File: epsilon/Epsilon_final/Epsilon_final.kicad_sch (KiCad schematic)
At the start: 16 parts, among them J3 Conn_01x02_Pin, J4 Conn_01x02_Pin, Q5 AO3401A, U12 ADA4940-1ARZ-R7, U8 DS28E07P+T

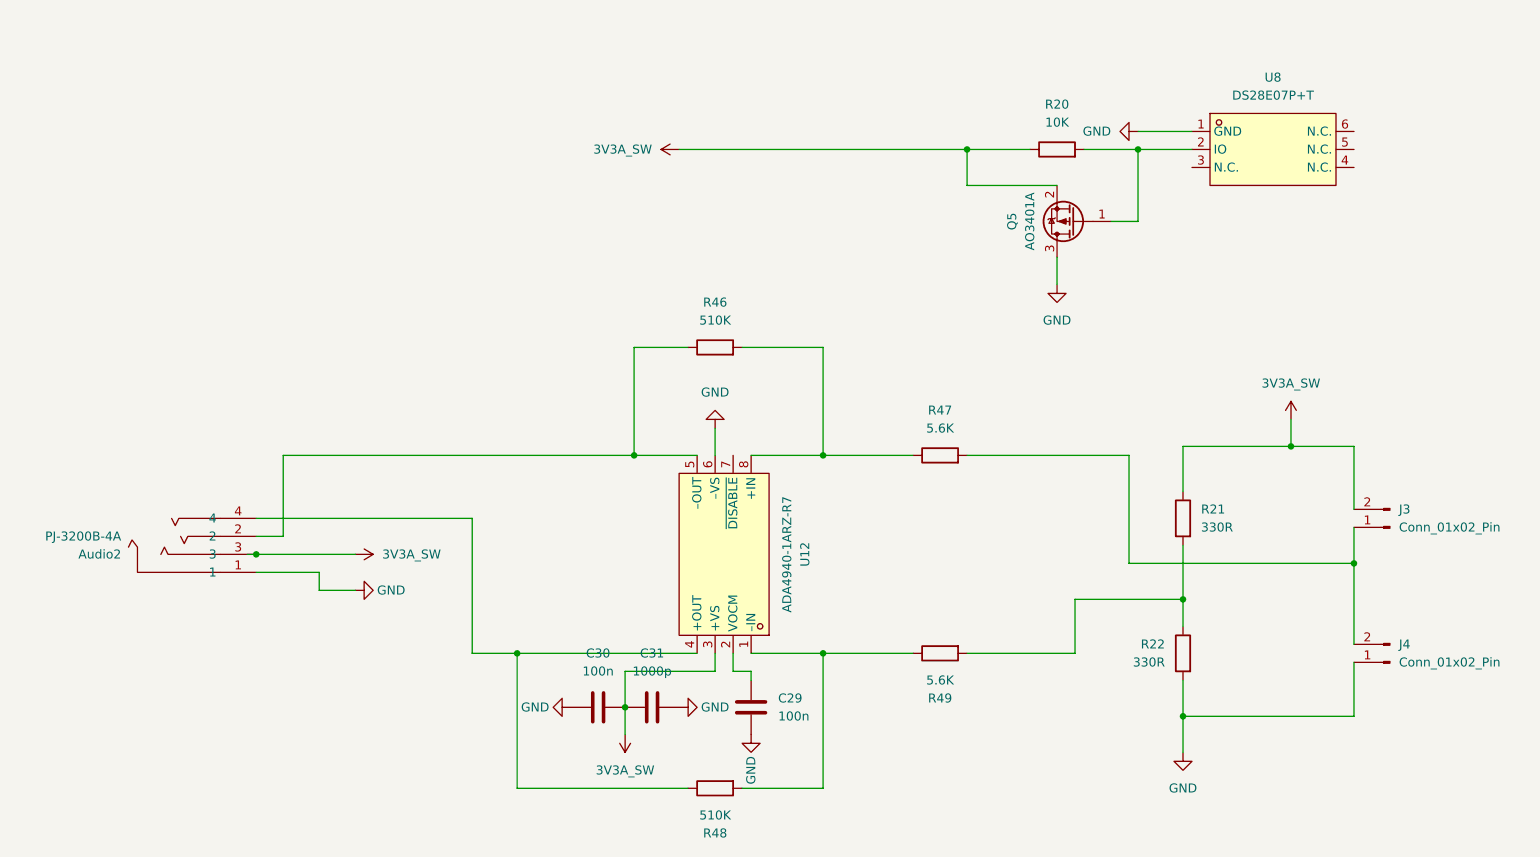
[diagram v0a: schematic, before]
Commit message: Yolo2
new Ozys
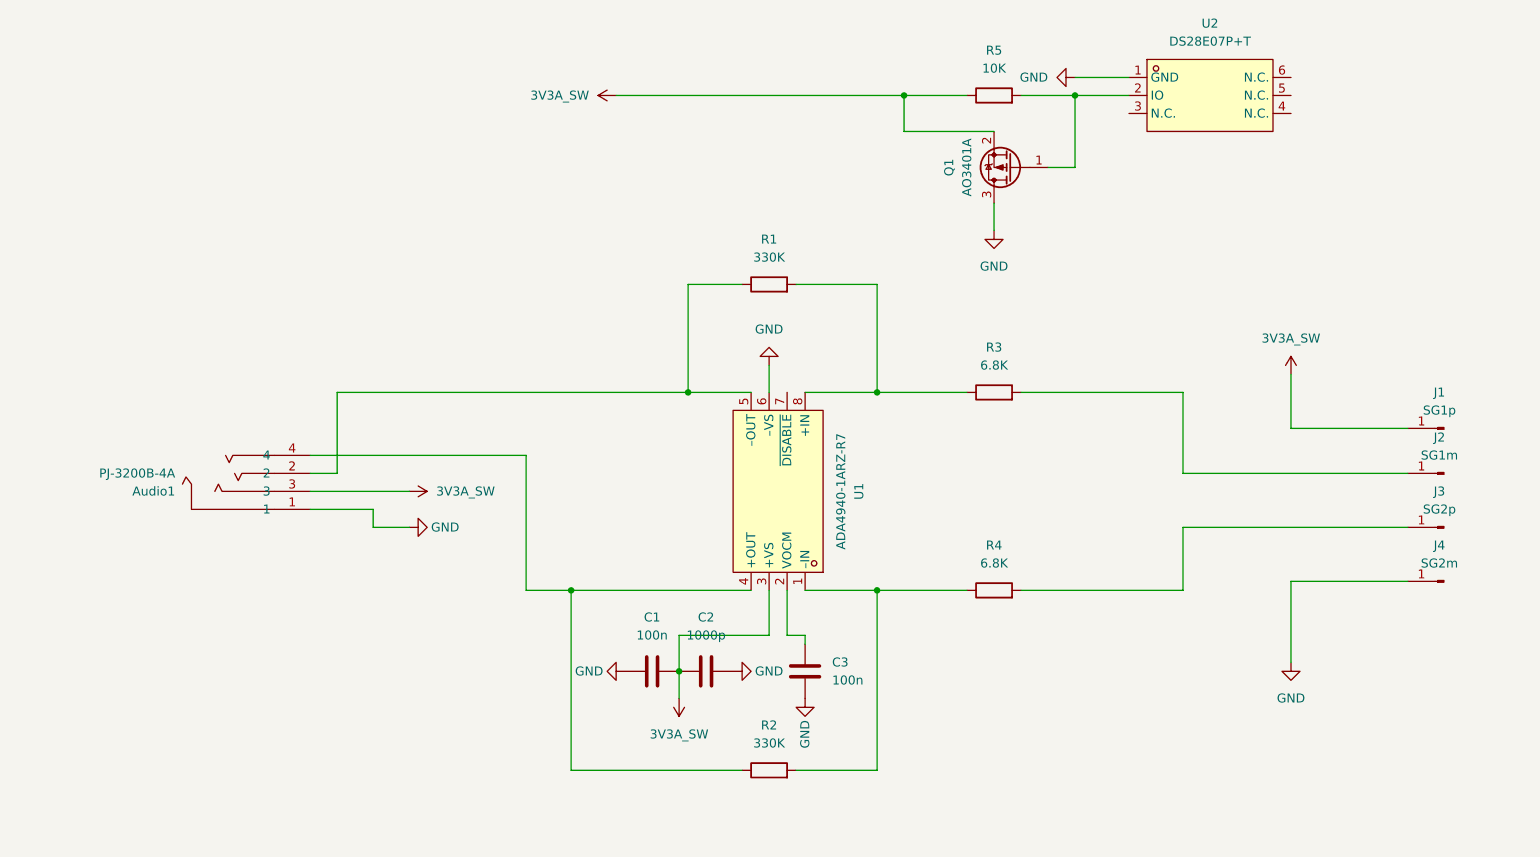
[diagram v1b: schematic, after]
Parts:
- removed Audio2: PJ-3200B-4A, Rocketry_Easyeda:AUDIO-TH_PJ-3200B-4A, symbol Rocketry_Easyeda:PJ-3200B-4A
- removed C29, C30: 100n, Capacitor_SMD:C_0402_1005Metric, symbol Device:C
- removed C31: 1000p, Capacitor_SMD:C_0402_1005Metric, symbol Device:C
- removed J3, J4: Conn_01x02_Pin, symbol Connector:Conn_01x02_Pin
- removed Q5: AO3401A, Package_TO_SOT_SMD:SOT-23, symbol Transistor_FET:AO3401A
- removed R20: 10K, symbol Device:R
- removed R21, R22: 330R, Resistor_SMD:R_0805_2012Metric_Pad1.20x1.40mm_HandSolder, symbol Device:R
- removed R46, R48: 510K, symbol Device:R
- removed R47, R49: 5.6K, symbol Device:R
- removed U12: ADA4940-1ARZ-R7, Rocketry_Easyeda:SOIC-8_L4.9-W3.9-P1.27-LS6.0-BL, symbol Rocketry_Easyeda:ADA4940-1ARZ-R7
- removed U8: DS28E07P+T, Rocketry_Easyeda:TSOC-6_L3.9-W4.3-P1.27-BL, symbol Rocketry_Easyeda:DS28E07P+T
- added Audio1: PJ-3200B-4A, Rocketry_Easyeda:AUDIO-TH_PJ-3200B-4A, symbol Rocketry_Easyeda:PJ-3200B-4A
- added C1, C3: 100n, Capacitor_SMD:C_0402_1005Metric, symbol Device:C
- added C2: 1000p, Capacitor_SMD:C_0402_1005Metric, symbol Device:C
- added J1: SG1p, Connector_Wire:SolderWirePad_1x01_SMD_1x2mm, symbol Connector:Conn_01x01_Pin
- added J2: SG1m, Connector_Wire:SolderWirePad_1x01_SMD_1x2mm, symbol Connector:Conn_01x01_Pin
- added J3: SG2p, Connector_Wire:SolderWirePad_1x01_SMD_1x2mm, symbol Connector:Conn_01x01_Pin
- added J4: SG2m, Connector_Wire:SolderWirePad_1x01_SMD_1x2mm, symbol Connector:Conn_01x01_Pin
- added Q1: AO3401A, Package_TO_SOT_SMD:SOT-23, symbol Transistor_FET:AO3401A
- added R1, R2: 330K, Resistor_SMD:R_0603_1608Metric_Pad0.98x0.95mm_HandSolder, symbol Device:R
- added R3, R4: 6.8K, Resistor_SMD:R_0603_1608Metric_Pad0.98x0.95mm_HandSolder, symbol Device:R
- added R5: 10K, Resistor_SMD:R_0402_1005Metric_Pad0.72x0.64mm_HandSolder, symbol Device:R
- added U1: ADA4940-1ARZ-R7, Rocketry_Easyeda:SOIC-8_L4.9-W3.9-P1.27-LS6.0-BL, symbol Rocketry_Easyeda:ADA4940-1ARZ-R7
- added U2: DS28E07P+T, Rocketry_Easyeda:TSOC-6_L3.9-W4.3-P1.27-BL, symbol Rocketry_Easyeda:DS28E07P+T
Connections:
- net 3V3A_SW: now also Audio1.3, C1.1, C2.2, J1.1 (Pin_1), Q1.2 (S), R5.1, U1.3 (+VS)
- net GND: now also Audio1.1, C1.2, C2.1, C3.1, J4.1 (Pin_1), Q1.3 (D), U1.6 (–VS), U2.1 (GND)
- new net: R1.2, R3.1, U1.8 (+IN)
- new net: J2.1 (Pin_1), R3.2
- new net: Q1.1 (G), R5.2, U2.2 (IO)
- new net: C3.2, U1.2 (VOCM)
- new net: R2.2, R4.1, U1.1 (–IN)
- new net: J3.1 (Pin_1), R4.2
- new net: Audio1.4, R2.1, U1.4 (+OUT)
- new net: Audio1.2, R1.1, U1.5 (–OUT)
